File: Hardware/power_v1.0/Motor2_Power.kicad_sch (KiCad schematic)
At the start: 16 parts, among them J1 Conn_01x02, U1 MP2338GTL-Z

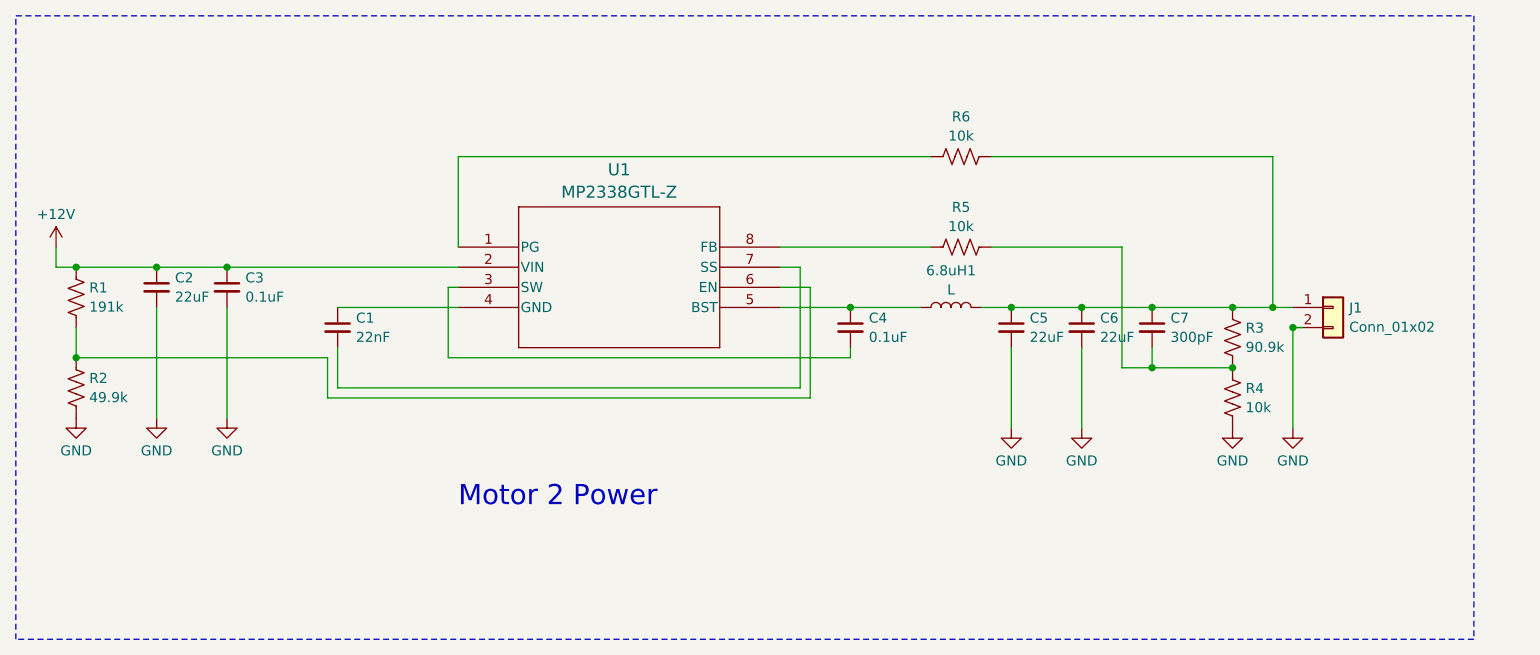
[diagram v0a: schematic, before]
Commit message: almost finished design of power board and working through design of brain board
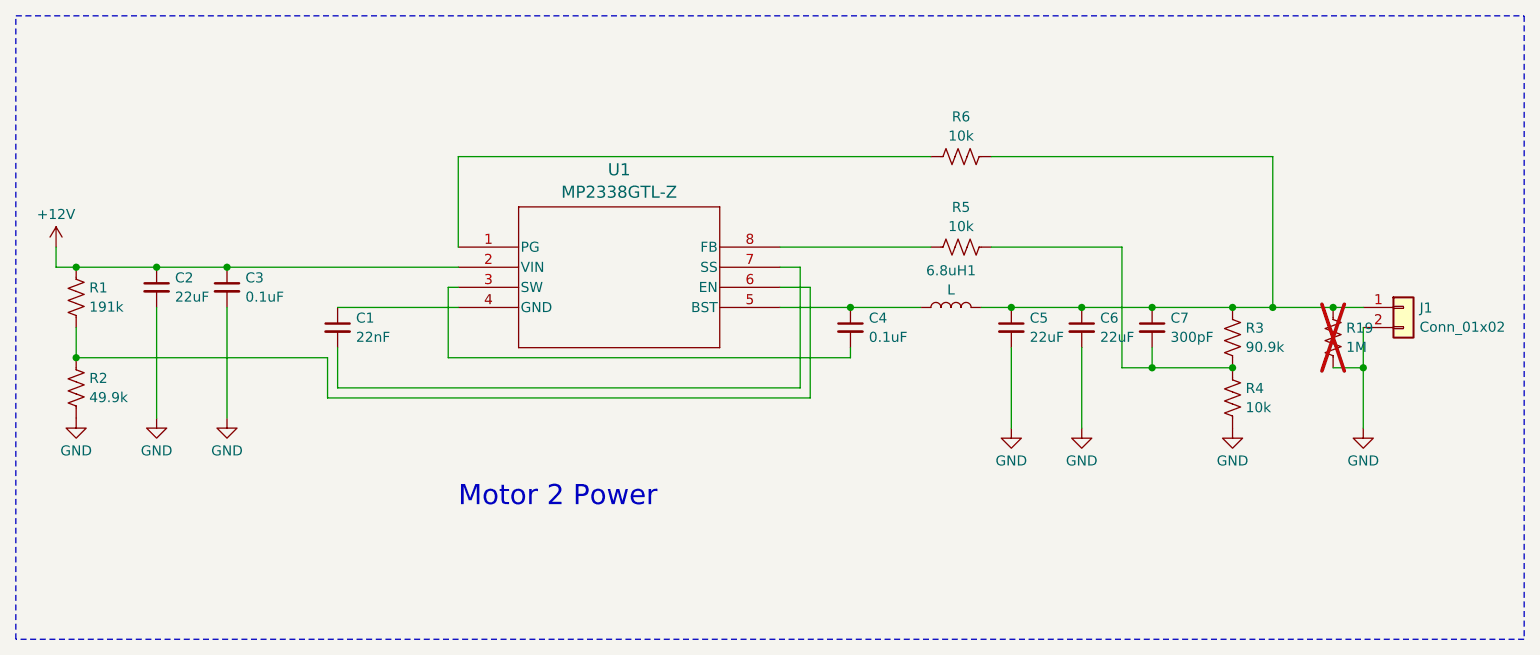
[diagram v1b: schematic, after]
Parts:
- added R19: 1M, symbol Device:R_US
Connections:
- net GND: now also R19.2
- net at 6.8uH1.2, C5.1, C6.1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: now also R19.1
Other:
- moved on the sheet: J1
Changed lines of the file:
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@@
     (company "By: Omkar Kulkarni")
   )
+  (junction (at 224.79 95.25) (diameter 0) (color 0 0 0 0)
+  )
   (junction (at 66.04 101.6) (diameter 0) (color 0 0 0 0)
   )
@@
   (junction (at 184.15 95.25) (diameter 0) (color 0 0 0 0)
   )
-  (junction (at 219.71 97.79) (diameter 0) (color 0 0 0 0)
-  )
   (junction (at 212.09 95.25) (diameter 0) (color 0 0 0 0)
   )
   (junction (at 66.04 90.17) (diameter 0) (color 0 0 0 0)
   )
+  (junction (at 228.6 102.87) (diameter 0) (color 0 0 0 0)
+  )
   (junction (at 217.17 95.25) (diameter 0) (color 0 0 0 0)
   )
@@
     (stroke (width 0) (type default))
   )
+  (wire (pts (xy 228.6 102.87) (xy 228.6 110.49))
+    (stroke (width 0) (type default))
+  )
   (wire (pts (xy 184.15 95.25) (xy 193.04 95.25))
     (stroke (width 0) (type default))
@@
     (stroke (width 0) (type default))
   )
-  (wire (pts (xy 217.17 95.25) (xy 219.71 95.25))
-    (stroke (width 0) (type default))
-  )
-  (wire (pts (xy 219.71 97.79) (xy 220.98 97.79))
+  (wire (pts (xy 217.17 95.25) (xy 224.79 95.25))
     (stroke (width 0) (type default))
   )
@@
     (stroke (width 0) (type default))
   )
-  (wire (pts (xy 219.71 97.79) (xy 219.71 110.49))
-    (stroke (width 0) (type default))
-  )
   (wire (pts (xy 217.17 76.2) (xy 217.17 95.25))
     (stroke (width 0) (type default))
@@
     (stroke (width 0) (type default))
   )
+  (wire (pts (xy 228.6 97.79) (xy 228.6 102.87))
+    (stroke (width 0) (type default))
+  )
   (wire (pts (xy 198.12 102.87) (xy 201.93 102.87))
     (stroke (width 0) (type default))
@@
     (stroke (width 0) (type default))
   )
+  (wire (pts (xy 224.79 95.25) (xy 228.6 95.25))
+    (stroke (width 0) (type default))
+  )
   (wire (pts (xy 76.2 90.17) (xy 85.09 90.17))
     (stroke (width 0) (type default))
@@
     (stroke (width 0) (type default))
   )
+  (wire (pts (xy 228.6 102.87) (xy 224.79 102.87))
+    (stroke (width 0) (type default))
+  )
   (wire (pts (xy 113.03 101.6) (xy 163.83 101.6))
     (stroke (width 0) (type default))
@@
     (stroke (width 0) (type default))
   )
-  (rectangle (start 58.42 58.42) (end 242.57 137.16)
+  (rectangle (start 58.42 58.42) (end 248.92 137.16)
     (stroke (width 0) (type dash))
     (fill (type none))
@@
     (effects (font (size 2.54 2.54)) (justify left bottom))
   )
-  (symbol (lib_id "power:GND") (at 219.71 110.49 0) (unit 1)
-    (in_bom yes) (on_board yes) (dnp no) (fields_autoplaced)
-    (property "Reference" "#PWR09" (at 219.71 116.84 0)
-      (effects (font (size 1.27 1.27)) hide)
-    )
-    (property "Value" "GND" (at 219.71 114.6231 0)
+  (symbol (lib_id "power:GND") (at 228.6 110.49 0) (unit 1)
+    (in_bom yes) (on_board yes) (dnp no) (fields_autoplaced)
+    (property "Reference" "#PWR09" (at 228.6 116.84 0)
+      (effects (font (size 1.27 1.27)) hide)
+    )
+    (property "Value" "GND" (at 228.6 114.6231 0)
       (effects (font (size 1.27 1.27)))
     )
-    (property "Footprint" "" (at 219.71 110.49 0)
-      (effects (font (size 1.27 1.27)) hide)
-    )
-    (property "Datasheet" "" (at 219.71 110.49 0)
+    (property "Footprint" "" (at 228.6 110.49 0)
+      (effects (font (size 1.27 1.27)) hide)
+    )
+    (property "Datasheet" "" (at 228.6 110.49 0)
       (effects (font (size 1.27 1.27)) hide)
     )
@@
     )
   )
-  (symbol (lib_id "Connector_Generic:Conn_01x02") (at 224.79 95.25 0) (unit 1)
-    (in_bom yes) (on_board yes) (dnp no) (fields_autoplaced)
-    (property "Reference" "J1" (at 226.822 95.3079 0)
-      (effects (font (size 1.27 1.27)) (justify left))
-    )
-    (property "Value" "Conn_01x02" (at 226.822 97.7321 0)
-      (effects (font (size 1.27 1.27)) (justify left))
-    )
-    (property "Footprint" "" (at 224.79 95.25 0)
-      (effects (font (size 1.27 1.27)) hide)
-    )
-    (property "Datasheet" "~" (at 224.79 95.25 0)
+  (symbol (lib_id "Connector_Generic:Conn_01x02") (at 233.68 95.25 0) (unit 1)
+    (in_bom yes) (on_board yes) (dnp no) (fields_autoplaced)
+    (property "Reference" "J1" (at 235.712 95.3079 0)
+      (effects (font (size 1.27 1.27)) (justify left))
+    )
+    (property "Value" "Conn_01x02" (at 235.712 97.7321 0)
+      (effects (font (size 1.27 1.27)) (justify left))
+    )
+    (property "Footprint" "" (at 233.68 95.25 0)
+      (effects (font (size 1.27 1.27)) hide)
+    )
+    (property "Datasheet" "~" (at 233.68 95.25 0)
       (effects (font (size 1.27 1.27)) hide)
     )
@@
         )
       )
+    )
+  )
+  (symbol (lib_id "Device:R_US") (at 224.79 99.06 0) (unit 1)
+    (in_bom yes) (on_board yes) (dnp yes) (fields_autoplaced)
+    (property "Reference" "R19" (at 226.441 97.8479 0)
+      (effects (font (size 1.27 1.27)) (justify left))
+    )
+    (property "Value" "1M" (at 226.441 100.2721 0)
+      (effects (font (size 1.27 1.27)) (justify left))
+    )
+    (property "Footprint" "" (at 225.806 99.314 90)
+      (effects (font (size 1.27 1.27)) hide)
+    )
+    (property "Datasheet" "~" (at 224.79 99.06 0)
+      (effects (font (size 1.27 1.27)) hide)
+    )
+    (pin "1")
+    (pin "2")
+    (instances
+      (project "power_v1.0"
+        (path "/1e1b062d-fad0-427c-a622-c5b8a80b5268/89921523-dfe0-4fb9-af02-a9673a087402"
+          (reference "R19") (unit 1)
+        )
+      )
